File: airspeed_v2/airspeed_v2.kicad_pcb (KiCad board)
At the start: 2 copper layers, 30 x 30 mm, 17 parts, among them J1 Conn_01x04_Pin, J3 Conn_01x02_Pin, U1 XGZP6897D, U2 MPU-9250, U3 SHT4x, U4 MS5611-01BA, U5 XGZP6897D, U6 BME280

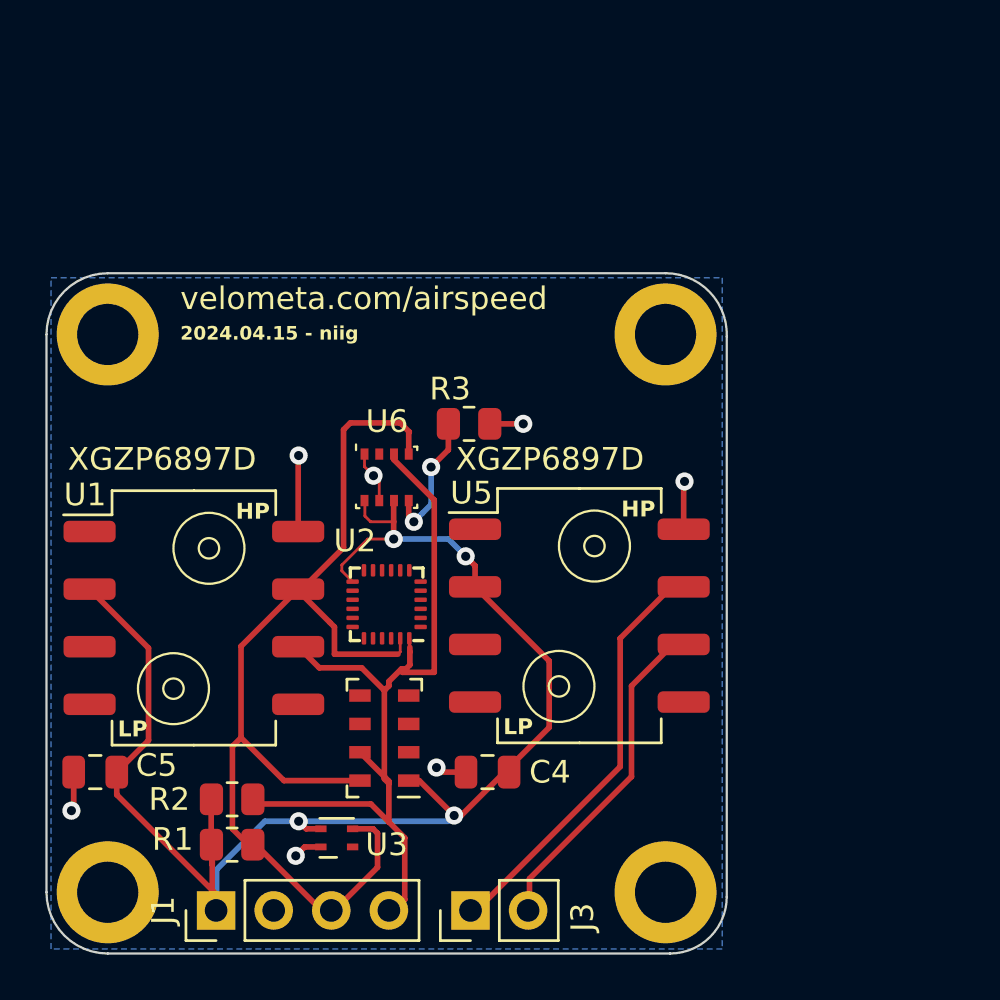
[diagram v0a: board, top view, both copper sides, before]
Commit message: airspeed v2
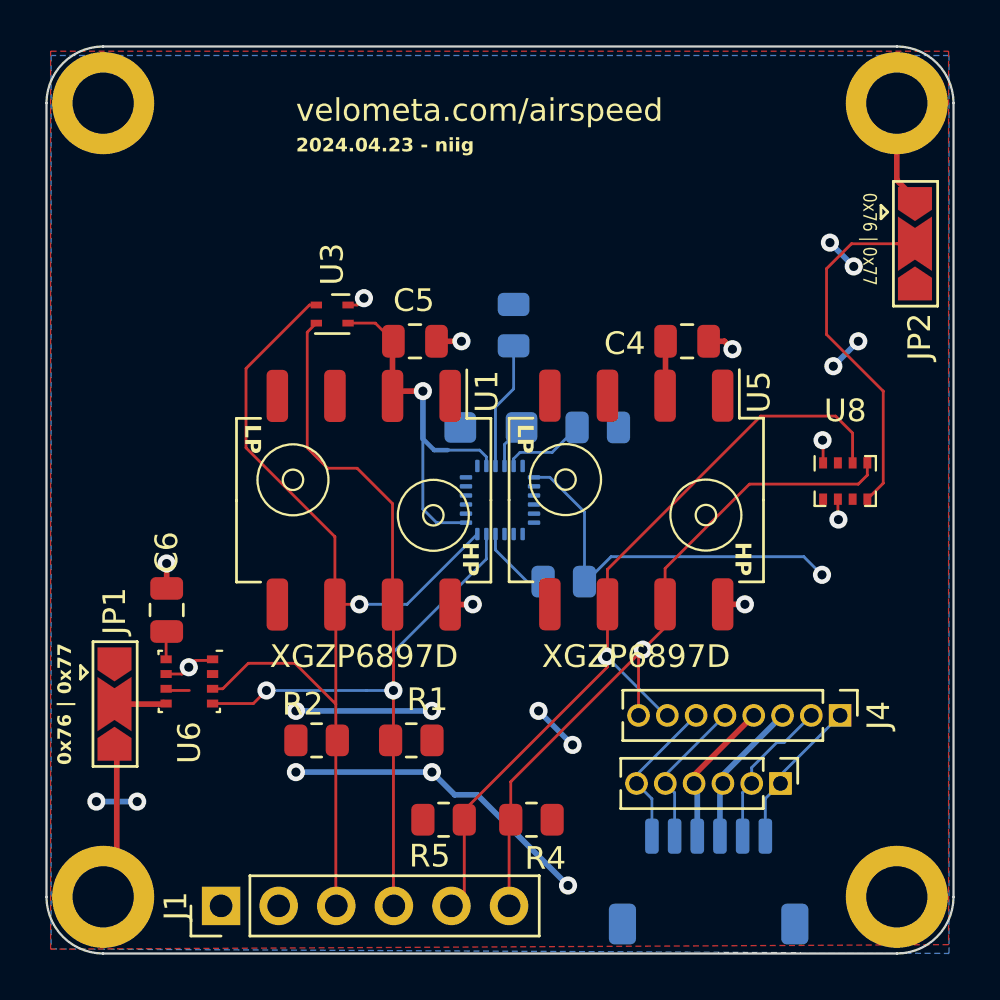
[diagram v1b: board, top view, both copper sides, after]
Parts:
- removed U4: MS5611-01BA, Package_LGA:LGA-8_3x5mm_P1.25mm
- added C6: C, Capacitor_SMD:C_0805_2012Metric, F.Cu at (65.3, 64.8)
- added C9: 0.1pF, Capacitor_Tantalum_SMD:CP_EIA-3216-18_Kemet-A, B.Cu at (79.6, 56.8)
- added J2: GPS, Connector_JST:JST_SH_SM06B-SRSS-TB_1x06-1MP_P1.00mm_Horizontal, B.Cu at (89.2, 76.8)
- added J4: ScreenIO, Connector_PinHeader_1.27mm:PinHeader_1x08_P1.27mm_Vertical, F.Cu at (95.0, 69.5)
- added JP1: 0x76 | 0x77, Jumper:SolderJumper-3_P2.0mm_Open_TrianglePad1.0x1.5mm, F.Cu at (63.0, 69.0)
- added JP2: 0x76 | 0x77, Jumper:SolderJumper-3_P2.0mm_Open_TrianglePad1.0x1.5mm, F.Cu at (98.3, 48.7)
- added R4: 10k, Resistor_SMD:R_0805_2012Metric, F.Cu at (81.4, 74.1)
- added R5: 10k, Resistor_SMD:R_0805_2012Metric, F.Cu at (77.5, 74.1)
- added R6: 10k, Resistor_SMD:R_0805_2012Metric, B.Cu at (80.6, 52.3)
- added R7: 10k, Resistor_SMD:R_0805_2012Metric, B.Cu at (82.8, 63.6)
- added U8: BMP280, Package_LGA:Bosch_LGA-8_2x2.5mm_P0.65mm_ClockwisePinNumbering, F.Cu at (95.2, 59.2)
- J1: value Conn_01x04_Pin -> Header; footprint Connector_PinHeader_2.54mm:PinHeader_1x04_P2.54mm_Vertical -> Connector_PinHeader_2.54mm:PinHeader_1x06_P2.54mm_Vertical
- J3: value Conn_01x02_Pin -> GPS; footprint Connector_PinHeader_2.54mm:PinHeader_1x02_P2.54mm_Vertical -> Connector_PinHeader_1.27mm:PinHeader_1x06_P1.27mm_Vertical
- R3, U2: moved to B.Cu
- moved C5 23.7 mm to (76.2, 53.0), turned to 0 degrees
- moved U3 23.1 mm to (72.6, 51.8), turned to 0 degrees
- moved C4 20.9 mm to (88.2, 53.0), turned to 0 degrees
- moved J3 14.8 mm to (92.4, 72.5), turned to -90 degrees
- moved H1 14.4 mm to (97.5, 42.5)
- moved U6 12.5 mm to (66.3, 68.0), turned to -90 degrees
- moved H2 10.2 mm to (62.5, 42.5)
- moved H4 10.2 mm to (97.5, 77.5)
- moved R1 9.14 mm to (76.1, 70.6), turned to 180 degrees
- moved U1 9.11 mm to (74.0, 60.0), turned to -90 degrees
- moved U2 6.79 mm to (80.0, 60.0), turned to 0 degrees
- moved U5 5.68 mm to (86.0, 60.0), turned to -90 degrees
- moved R3 5.68 mm to (84.3, 56.8)
- moved R2 4.54 mm to (71.9, 70.6)
- moved J1 0.30 mm to (67.7, 77.9)
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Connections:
- C4 pad 1: 3v3 -> +3V3
- C5 pad 1: 3v3 -> +3V3
- J1 pad 1: 3v3 -> +3V3
- J1 pad 3: SCL -> SDA
- J1 pad 4: SDA -> SCL
- J3 pad 1: SCL2 -> Rx
- J3 pad 2: SDA2 -> Tx
- R1 pad 1: 3v3 -> +3V3
- R2 pad 1: 3v3 -> +3V3
- R3 pad 1: Net-(U6-SDO) -> Net-(U2-FSYNC)
- U1 pad 2: 3v3 -> +3V3
- U2 pad 1: unconnected-(U2-RESV_VDDIO-Pad1) -> +3V3
- U2 pad 10: unconnected-(U2-REGOUT-Pad10) -> Net-(U2-REGOUT)
- U2 pad 11: unconnected-(U2-FSYNC-Pad11) -> Net-(U2-FSYNC)
- U2 pad 13: 3v3 -> +3V3
- U2 pad 20: unconnected-(U2-RESV_GND-Pad20) -> GND
- U2 pad 22: unconnected-(U2-~{CS}-Pad22) -> Net-(U2-~{CS})
- U2 pad 8: unconnected-(U2-VDDIO-Pad8) -> +3V3
- U2 pad 9: unconnected-(U2-AD0/MISO-Pad9) -> Net-(U2-AD0/MISO)
- U3 pad 3: 3v3 -> +3V3
- U5 pad 2: 3v3 -> +3V3
- U6 pad 2: unconnected-(U6-CSB-Pad2) -> +3V3
- U6 pad 5: Net-(U6-SDO) -> Net-(JP1-C)
- U6 pad 6: 3v3 -> +3V3
- U6 pad 8: 3v3 -> +3V3
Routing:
- net 3v3: track 66.9 -> 0.00 mm, vias 4 -> 0
- net +3V3: track 0.00 -> 66.2 mm, vias 0 -> 15
- net SDA2: track 15.0 -> 36.7 mm, vias 0 -> 1
- net Net-(JP2-C): track 0.00 -> 16.6 mm
- net GND: track 13.5 -> 29.3 mm, vias 7 -> 9
- net SCL2: track 18.6 -> 31.9 mm, vias 0 -> 1
- net SDA: track 38.9 -> 50.7 mm, vias 0 -> 1
- net Tx: track 0.00 -> 6.77 mm
- net Rx: track 0.00 -> 6.69 mm
- net 5V: track 0.00 -> 6.47 mm
- net Net-(U6-SDO): track 6.16 -> 0.00 mm, vias 2 -> 0
- net Net-(U2-AD0/MISO): track 0.00 -> 5.63 mm
- net Net-(U2-FSYNC): track 0.00 -> 3.69 mm
- net Net-(U2-~{CS}): track 0.00 -> 3.38 mm
- net SCL: track 48.5 -> 51.7 mm, vias 0 -> 2
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- added copper zone on F.Cu, net +3V3
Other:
- board size 30 x 30 mm -> 40 x 40 mm
- board text added: "2024.04.23 - niig"
- board text removed: "2024.04.15 - niig"
